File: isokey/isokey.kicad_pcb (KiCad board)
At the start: 2 copper layers, 336 parts, among them J1 PadExp Right, J2 PadExp Left, Q1 BSS138, SW1 Cherry, SW10 Cherry, SW11 Cherry, SW12 Cherry, SW13 Cherry, SW14 Cherry, SW15 Cherry, SW16 Cherry, SW17 Cherry, SW18 Cherry, SW19 Cherry, SW2 Cherry, SW20 Cherry, SW21 Cherry, SW22 Cherry, SW23 Cherry, SW24 Cherry, SW25 Cherry, SW26 Cherry, SW27 Cherry, SW28 Cherry, SW29 Cherry, SW3 Cherry, SW30 Cherry, SW31 Cherry, SW32 Cherry, SW33 Cherry, SW34 Cherry, SW35 Cherry, SW36 Cherry, SW37 Cherry, SW38 Cherry, SW39 Cherry, SW4 Cherry, SW40 Cherry, SW41 Cherry, SW42 Cherry, SW43 Cherry, SW44 Cherry, SW45 Cherry, SW46 Cherry, SW47 Cherry, SW48 Cherry, SW5 Cherry, SW6 Cherry, SW7 Cherry, SW8 Cherry, SW9 Cherry, U1 BlackPill_STLINK, U3 TLV73318PDBV, U4 LP5569

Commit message: Continue routing
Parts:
- removed C38, C63, C64, C65, C66, C67, C68, C69, C70, C71, C72, C73, C74, C75, C76, C77, C78, C79, C80, C81, C82, C83: 100nF, Capacitor_SMD:C_0603_1608Metric_Pad1.08x0.95mm_HandSolder
- removed D100, D74, D79, D80, D81, D82, D83, D84, D85, D86, D87, D88, D89, D90, D91, D92, D93, D94, D95, D96, D97, D98, D99: SK6812MINI, LED_SMD:LED_SK6812MINI_PLCC4_3.5x3.5mm_P1.75mm
- removed the U1 at (190.0, -37.0)
- removed the U1 at (168.5, -38.0)
- added U1: BlackPill_STLINK, Module:BlackPill_doble_top-bot, F.Cu at (222.4, -40.8)
- C15, C16, C18, C19, C21, C22, C24, C25, C28, C32, C33, C39, C42, C45, C48, C51, C52, C54, C55, C56, C61, C62, D119, D26, D28: moved to B.Cu
- D27, D29: moved to F.Cu
- D30, D32, D34, D36, D38, D40, D41, D42, D44, D48, D50, D52, D54, D56, D58, D60, D62, D64, D66, D68, D72, D75, D76, D78: value SK6812MINI -> SK6812MINI-E; moved to B.Cu
- D31, D33, D35, D37, D39, D43, D45, D46, D47, D49, D51, D53, D55, D57, D59, D61, D63, D65, D67, D69, D70, D71, D73, D77: value SK6812MINI -> SK6812MINI-E
- moved R38 329.8 mm to (196.4, 10.5)
- moved R39 329.0 mm to (196.6, 12.3)
- moved C8 317.0 mm to (203.5, 13.8), turned to 180 degrees
- moved R33 312.3 mm to (209.4, 13.8)
- moved R40 309.7 mm to (201.3, -5.71)
- moved C9 309.6 mm to (209.4, 11.3)
- moved R35 309.4 mm to (203.5, 11.3)
- moved C10 277.6 mm to (191.9, -13.9)
- moved C11 277.6 mm to (191.9, -10.9)
- moved C12 277.6 mm to (191.9, -7.84)
- moved C13 277.6 mm to (191.9, -4.83)
- moved U3 277.6 mm to (202.4, -14.7)
- moved R31 273.0 mm to (236.6, -20.5), turned to 180 degrees
- moved R18 271.0 mm to (240.1, -25.6), turned to 180 degrees
- moved R20 268.8 mm to (240.1, -23.0), turned to 180 degrees
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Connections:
- D31 pad 1: Net-(D31-DOUT) -> Net-(D30-DOUT)
- D31 pad 3: Net-(D30-DOUT) -> Net-(D30-DIN)
- D32 pad 3: Net-(D31-DOUT) -> Net-(D30-DOUT)
- D33 pad 1: Net-(D33-DOUT) -> Net-(D32-DOUT)
- D33 pad 3: Net-(D32-DOUT) -> Net-(D30-DOUT)
- D34 pad 3: Net-(D33-DOUT) -> Net-(D32-DOUT)
- D35 pad 1: Net-(D35-DOUT) -> Net-(D34-DOUT)
- D35 pad 3: Net-(D34-DOUT) -> Net-(D32-DOUT)
- D36 pad 3: Net-(D35-DOUT) -> Net-(D34-DOUT)
- D37 pad 1: Net-(D37-DOUT) -> Net-(D36-DOUT)
- D37 pad 3: Net-(D36-DOUT) -> Net-(D34-DOUT)
- D38 pad 3: Net-(D37-DOUT) -> Net-(D36-DOUT)
- D39 pad 1: Net-(D39-DOUT) -> Net-(D38-DOUT)
- D39 pad 3: Net-(D38-DOUT) -> Net-(D36-DOUT)
- D40 pad 3: Net-(D39-DOUT) -> Net-(D38-DOUT)
- D45 pad 1: Net-(D45-DOUT) -> Net-(D40-DOUT)
- D45 pad 3: Net-(D44-DOUT) -> Net-(D38-DOUT)
- D46 pad 1: Net-(D46-DOUT) -> Net-(D41-DOUT)
- D46 pad 3: Net-(D45-DOUT) -> Net-(D40-DOUT)
- D47 pad 1: Net-(D47-DOUT) -> Net-(D42-DOUT)
- D47 pad 3: Net-(D46-DOUT) -> Net-(D41-DOUT)
- D48 pad 1: Net-(D48-DOUT) -> Net-(D43-DOUT)
- D48 pad 3: Net-(D47-DOUT) -> Net-(D42-DOUT)
- D49 pad 1: Net-(D49-DOUT) -> Net-(D44-DOUT)
- D49 pad 3: Net-(D48-DOUT) -> Net-(D43-DOUT)
- D50 pad 3: Net-(D49-DOUT) -> Net-(D44-DOUT)
- D55 pad 1: Net-(D55-DOUT) -> Net-(D50-DOUT)
- D55 pad 3: Net-(D54-DOUT) -> Net-(D44-DOUT)
- D56 pad 1: Net-(D56-DOUT) -> Net-(D51-DOUT)
- D56 pad 3: Net-(D55-DOUT) -> Net-(D50-DOUT)
- D57 pad 1: Net-(D57-DOUT) -> Net-(D52-DOUT)
- D57 pad 3: Net-(D56-DOUT) -> Net-(D51-DOUT)
- D58 pad 1: Net-(D58-DOUT) -> Net-(D53-DOUT)
- D58 pad 3: Net-(D57-DOUT) -> Net-(D52-DOUT)
- D59 pad 1: Net-(D59-DOUT) -> Net-(D54-DOUT)
- D59 pad 3: Net-(D58-DOUT) -> Net-(D53-DOUT)
- D60 pad 3: Net-(D59-DOUT) -> Net-(D54-DOUT)
- D65 pad 1: Net-(D65-DOUT) -> Net-(D60-DOUT)
- D65 pad 3: Net-(D64-DOUT) -> Net-(D54-DOUT)
- D66 pad 1: Net-(D66-DOUT) -> Net-(D61-DOUT)
- D66 pad 3: Net-(D65-DOUT) -> Net-(D60-DOUT)
- D67 pad 1: Net-(D67-DOUT) -> Net-(D62-DOUT)
- D67 pad 3: Net-(D66-DOUT) -> Net-(D61-DOUT)
- D68 pad 1: Net-(D68-DOUT) -> Net-(D63-DOUT)
- D68 pad 3: Net-(D67-DOUT) -> Net-(D62-DOUT)
- D69 pad 1: Net-(D69-DOUT) -> Net-(D64-DOUT)
- D69 pad 3: Net-(D68-DOUT) -> Net-(D63-DOUT)
- D70 pad 3: Net-(D69-DOUT) -> Net-(D64-DOUT)
- D73 pad 1: Net-(D73-DOUT) -> /led_w1_out
- D75 pad 1: Net-(D75-DOUT) -> Net-(D70-DOUT)
- D75 pad 3: Net-(D74-DOUT) -> Net-(D64-DOUT)
- D76 pad 1: Net-(D76-DOUT) -> Net-(D71-DOUT)
- D76 pad 3: Net-(D75-DOUT) -> Net-(D70-DOUT)
- D77 pad 1: Net-(D77-DOUT) -> Net-(D72-DOUT)
- D77 pad 3: Net-(D76-DOUT) -> Net-(D71-DOUT)
- D78 pad 1: Net-(D78-DOUT) -> /led_w1_out
- D78 pad 3: Net-(D77-DOUT) -> Net-(D72-DOUT)
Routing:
- net GND: track 0.00 -> 826.7 mm, vias 0 -> 93
- net +5V: track 0.00 -> 746.9 mm, vias 0 -> 46
- net /cl3: track 0.00 -> 129.6 mm, vias 0 -> 9
- net /cl4: track 0.00 -> 124.9 mm, vias 0 -> 9
- net /sw0_r: track 0.00 -> 100.7 mm, vias 0 -> 7
- net /cl1: track 0.00 -> 100.7 mm, vias 0 -> 7
- net /cl2: track 0.00 -> 99.1 mm, vias 0 -> 7
- net /r0: track 0.00 -> 98.1 mm, vias 0 -> 5
- net /r3: track 0.00 -> 98.0 mm, vias 0 -> 5
- net /r1: track 0.00 -> 98.0 mm, vias 0 -> 5
- net /r2: track 0.00 -> 90.1 mm, vias 0 -> 5
- net +3.3V: track 0.00 -> 37.0 mm
- net Net-(D72-DOUT): track 0.00 -> 25.8 mm, vias 0 -> 3
- net Net-(D63-DOUT): track 0.00 -> 25.3 mm, vias 0 -> 4
- net Net-(D62-DOUT): track 0.00 -> 25.3 mm, vias 0 -> 4
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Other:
- board outline added: 4.6 x 4.6 mm

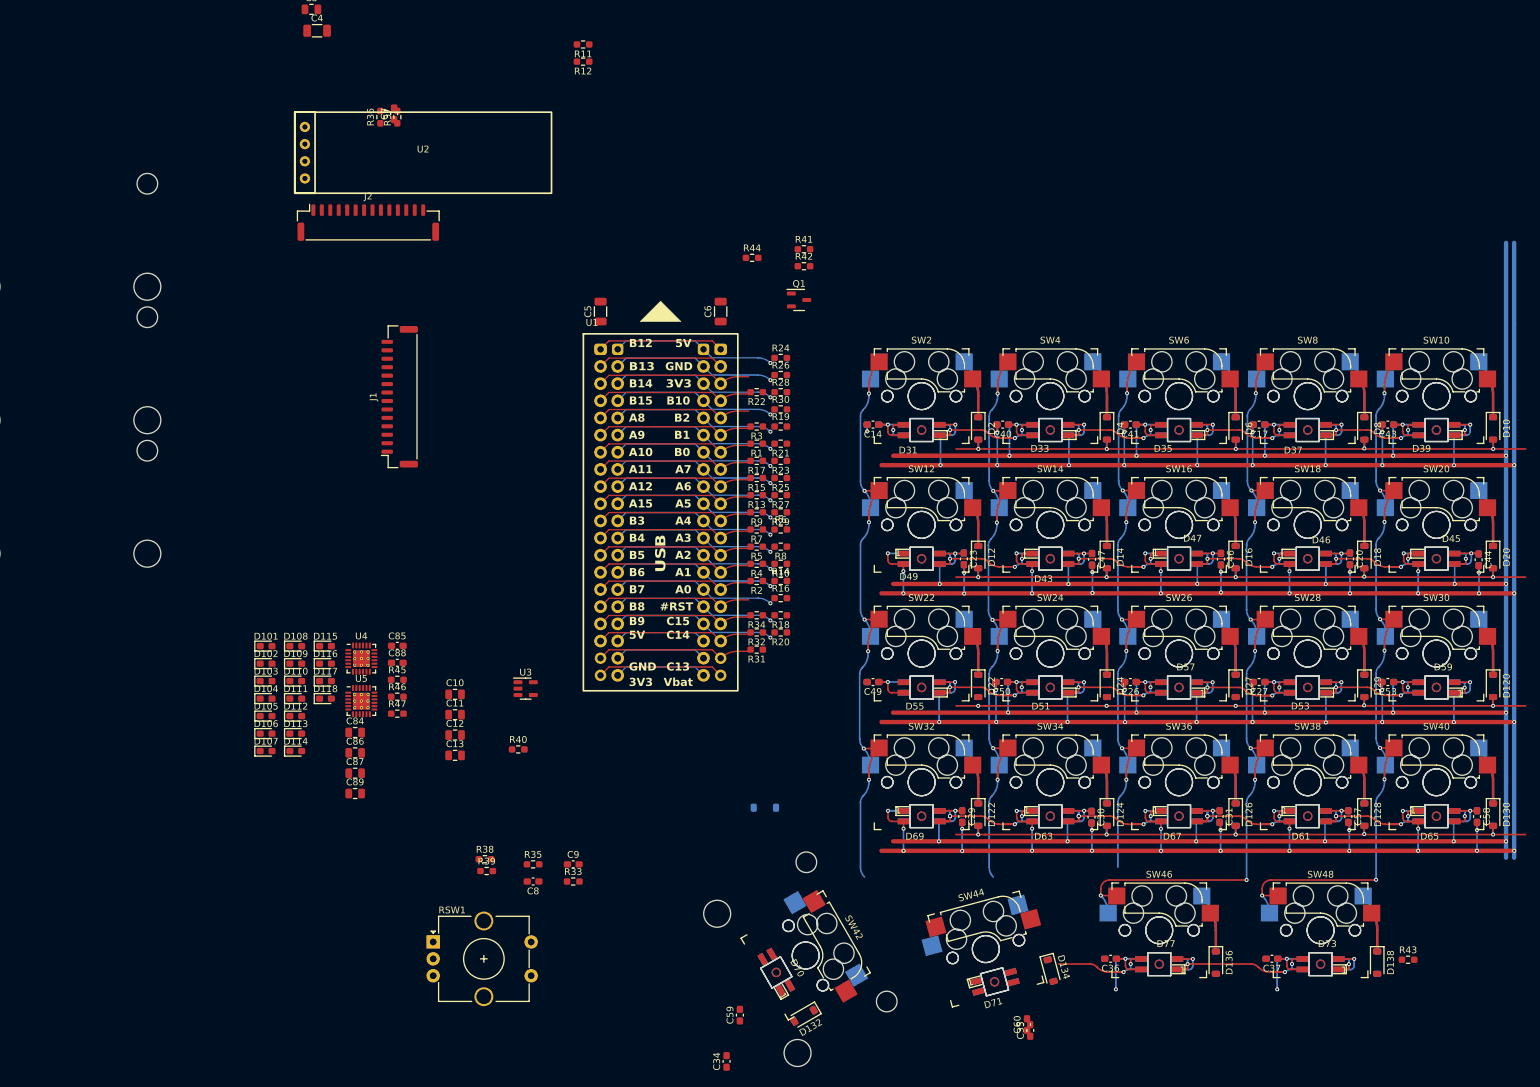
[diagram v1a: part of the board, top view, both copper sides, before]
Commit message: Continue routing
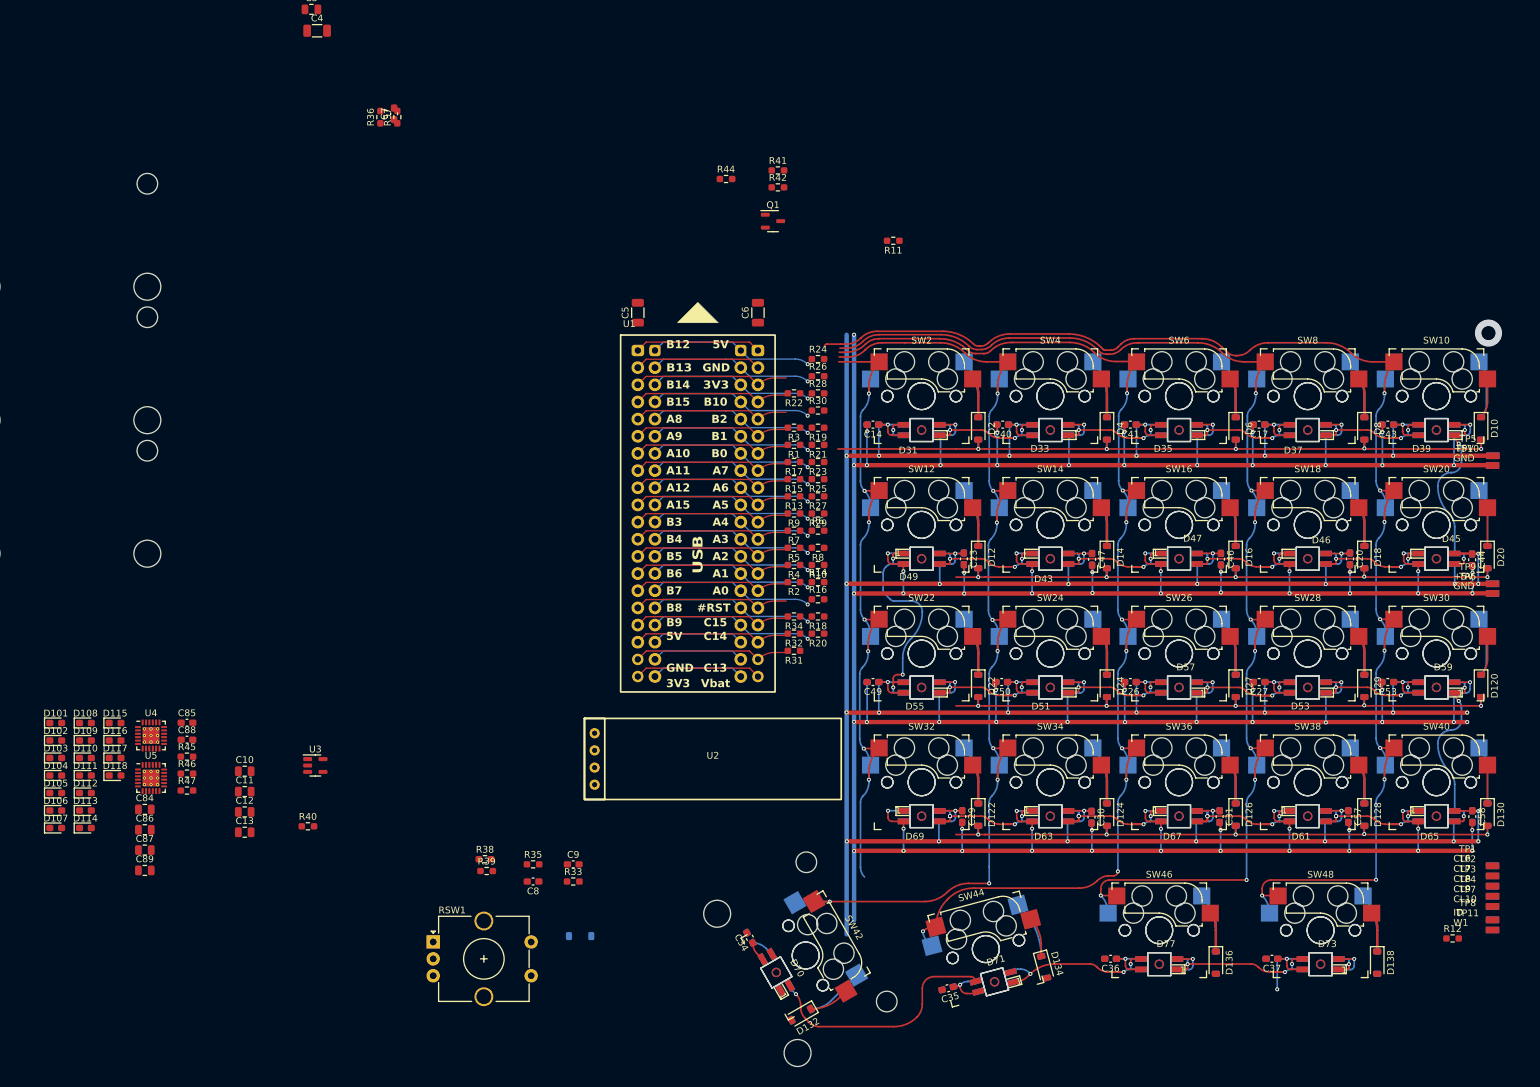
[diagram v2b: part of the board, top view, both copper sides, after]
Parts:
- removed J1: PadExp Right, Connector_JST:JST_GH_SM14B-GHS-TB_1x14-1MP_P1.25mm_Horizontal
- removed J2: PadExp Left, Connector_JST:JST_GH_SM14B-GHS-TB_1x14-1MP_P1.25mm_Horizontal
- removed R43: 22R, Resistor_SMD:R_0603_1608Metric_Pad0.98x0.95mm_HandSolder
- added TP1: CL6, TestPoint:Testpoint_Pad_1.0x2.0mm, F.Cu at (345.5, 11.5)
- added TP10: GND, TestPoint:Testpoint_Pad_1.0x2.0mm, F.Cu at (345.5, -47.7)
- added TP11: W1, TestPoint:Testpoint_Pad_1.0x2.0mm, F.Cu at (345.5, 21.0)
- added TP2: CL7, TestPoint:Testpoint_Pad_1.0x2.0mm, F.Cu at (345.5, 13.0)
- added TP3: CL8, TestPoint:Testpoint_Pad_1.0x2.0mm, F.Cu at (345.5, 14.5)
- added TP4: CL9, TestPoint:Testpoint_Pad_1.0x2.0mm, F.Cu at (345.5, 16.0)
- added TP5: +5V, TestPoint:Testpoint_Pad_1.0x2.0mm, F.Cu at (345.6, -49.2)
- added TP6: GND, TestPoint:Testpoint_Pad_1.0x2.0mm, F.Cu at (345.5, -28.8)
- added TP7: CL10, TestPoint:Testpoint_Pad_1.0x2.0mm, F.Cu at (345.5, 17.5)
- added TP8: ID, TestPoint:Testpoint_Pad_1.0x2.0mm, F.Cu at (345.5, 19.5)
- added TP9: +5V, TestPoint:Testpoint_Pad_1.0x2.0mm, F.Cu at (345.5, -30.2)
- C59, C60: moved to B.Cu
- moved R12 182.8 mm to (339.6, 22.3), turned to 0 degrees
- moved U2 99.5 mm to (230.1, -4.30)
- moved R11 54.3 mm to (256.8, -81.0)
- moved D131 37.5 mm to (243.2, 33.5), turned to -150 degrees
- moved D133 36.3 mm to (279.1, 26.5), turned to -75 degrees
- moved D25 33.3 mm to (210.4, 21.9)
- moved C85 33.1 mm to (152.3, -9.66)
- moved C88 33.1 mm to (152.3, -7.15)
- moved D115 33.1 mm to (141.6, -9.62)
- moved D116 33.1 mm to (141.6, -7.03)
- moved D117 33.1 mm to (141.6, -4.44)
- moved D118 33.1 mm to (141.6, -1.85)
- moved R40 33.1 mm to (170.2, 5.67)
- moved R45 33.1 mm to (152.3, -4.64)
- moved R46 33.1 mm to (152.3, -2.13)
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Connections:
- R12 pad 2: /port_id -> /led_w1_out
- R13 pad 1: /cl9 -> unconnected-(R13-Pad1)
- R15 pad 1: /cl10 -> unconnected-(R15-Pad1)
- R17 pad 1: /cl11 -> unconnected-(R17-Pad1)
- R19 pad 1: /r0 -> unconnected-(R19-Pad1)
- R2 pad 1: /cl4 -> unconnected-(R2-Pad1)
- R21 pad 1: /r1 -> unconnected-(R21-Pad1)
- R23 pad 1: /r2 -> unconnected-(R23-Pad1)
- R24 pad 2: /~{CS} -> unconnected-(R24-Pad2)
- R25 pad 1: /r3 -> unconnected-(R25-Pad1)
- R26 pad 2: /SCLK -> unconnected-(R26-Pad2)
- R27 pad 1: /r4 -> unconnected-(R27-Pad1)
- R28 pad 2: /MISO -> unconnected-(R28-Pad2)
- R29 pad 1: /r-1 -> unconnected-(R29-Pad1)
- R30 pad 2: /MOSI -> /r0
- R31 pad 1: /cl1 -> unconnected-(R31-Pad1)
- R32 pad 1: /cl2 -> unconnected-(R32-Pad1)
- R34 pad 1: /cl3 -> unconnected-(R34-Pad1)
- R4 pad 1: /cl5 -> unconnected-(R4-Pad1)
- R5 pad 1: /cl6 -> unconnected-(R5-Pad1)
- R7 pad 1: /cl7 -> unconnected-(R7-Pad1)
- R9 pad 1: /cl8 -> unconnected-(R9-Pad1)
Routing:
- net /cl4: track 124.9 -> 213.9 mm
- net /cl2: track 99.1 -> 181.7 mm, vias 7 -> 9
- net /cl3: track 129.6 -> 195.8 mm
- net /cl1: track 100.7 -> 159.6 mm, vias 7 -> 9
- net Net-(D70-DOUT): track 0.00 -> 36.5 mm, vias 0 -> 1
- net +5V: track 746.9 -> 781.2 mm, vias 46 -> 51
- net Net-(D44-DOUT): track 0.00 -> 33.5 mm, vias 0 -> 3
- net Net-(D38-DOUT): track 8.77 -> 29.0 mm, vias 2 -> 3
- net Net-(D54-DOUT): track 8.77 -> 28.8 mm, vias 2 -> 3
- net /r0: track 98.1 -> 109.0 mm
- net Net-(D71-DOUT): track 16.6 -> 27.2 mm, vias 2 -> 3
- net Net-(D131-K): track 0.00 -> 8.66 mm
- net Net-(D133-K): track 0.00 -> 8.55 mm
- net Net-(D132-K): track 0.00 -> 6.02 mm
- net /sw0_r: track 100.7 -> 106.7 mm
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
